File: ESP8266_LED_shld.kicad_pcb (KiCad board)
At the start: 2 copper layers, 59.1 x 52.7 mm, 29 parts, among them J1 Pwr_Dat_Out, J2 CONN_02X08, J3 CONN_DIN, J4 BARREL_JACK, J5 USB-MICROB, J6 CONN_01X06, M1 LOGIC_LEVEL_CONVERTER, T1 Test_Point_2Pads, U1 ESP-07v2, U2 AMS1117

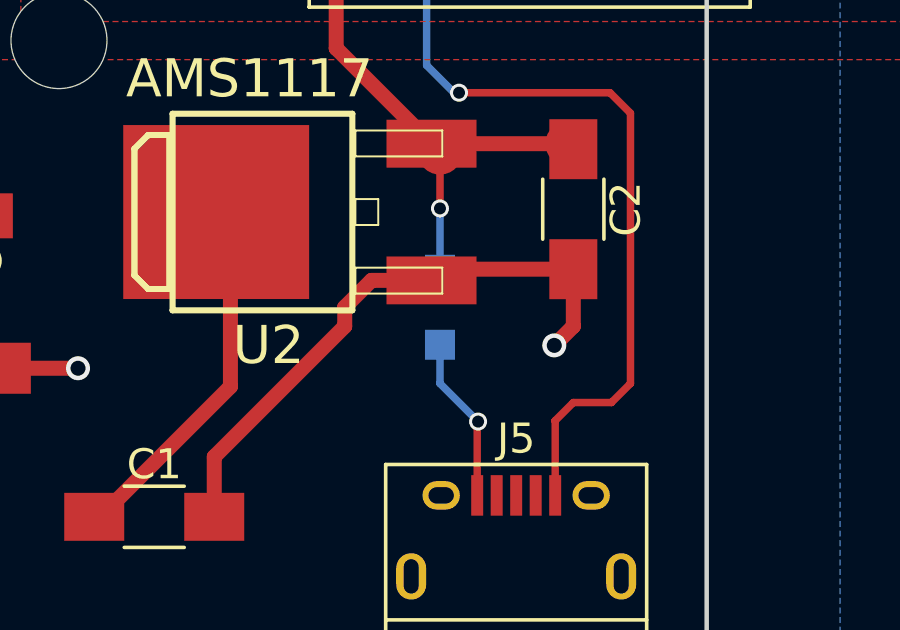
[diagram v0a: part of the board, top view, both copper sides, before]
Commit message: updated PCB design
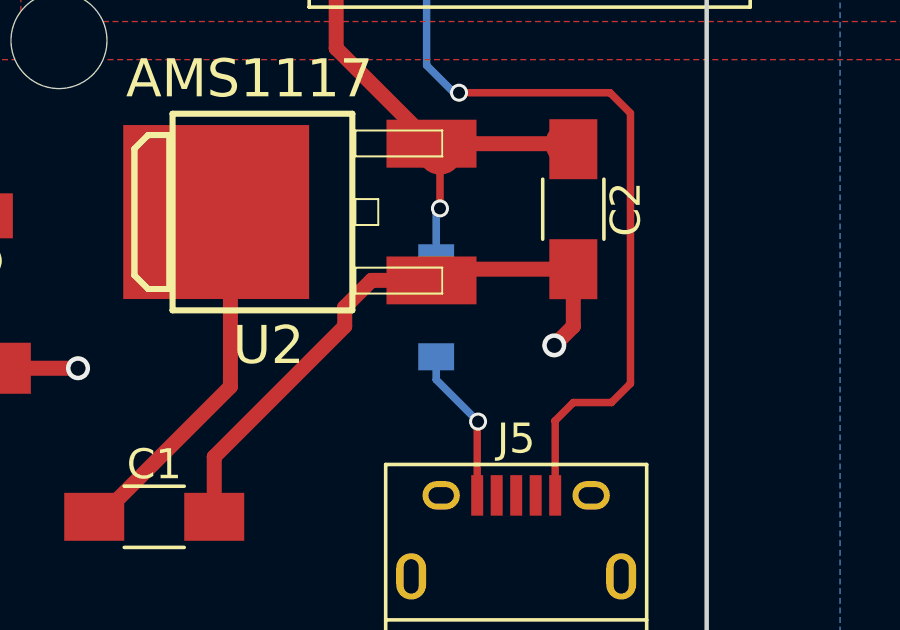
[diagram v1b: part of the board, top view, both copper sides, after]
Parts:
- D2: footprint Diodes_SMD:D_SOD-323_HandSoldering -> Diodes_SMD:D_SOD-123
- moved D2 0.13 mm to (208.8, 121.9)
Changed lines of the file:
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@@
     (thickness 1.6)
     (drawings 27)
-    (tracks 250)
+    (tracks 251)
     (zones 0)
     (modules 29)
@@
     )
   )
-  (module Diodes_SMD:D_SOD-323_HandSoldering (layer B.Cu)
-    (at 208.915 121.92 270)
-    (descr SOD-323)
-    (tags SOD-323)
-    (attr smd)
-    (fp_text reference D2 (at 0 1.85 270) (layer B.SilkS)
-      (effects (font (size 1 1) (thickness 0.15)) (justify mirror))
-    )
-    (fp_text value DIODE (at 0.1 -1.9 270) (layer B.Fab)
-      (effects (font (size 1 1) (thickness 0.15)) (justify mirror))
-    )
-    (fp_line (start -1.9 0.85) (end -1.9 -0.85) (layer B.SilkS) (width 0.12))
-    (fp_line (start 0.2 0) (end 0.45 0) (layer B.Fab) (width 0.1))
-    (fp_line (start 0.2 -0.35) (end -0.3 0) (layer B.Fab) (width 0.1))
-    (fp_line (start 0.2 0.35) (end 0.2 -0.35) (layer B.Fab) (width 0.1))
-    (fp_line (start -0.3 0) (end 0.2 0.35) (layer B.Fab) (width 0.1))
-    (fp_line (start -0.3 0) (end -0.5 0) (layer B.Fab) (width 0.1))
-    (fp_line (start -0.3 0.35) (end -0.3 -0.35) (layer B.Fab) (width 0.1))
-    (fp_line (start -0.9 -0.7) (end -0.9 0.7) (layer B.Fab) (width 0.1))
-    (fp_line (start 0.9 -0.7) (end -0.9 -0.7) (layer B.Fab) (width 0.1))
-    (fp_line (start 0.9 0.7) (end 0.9 -0.7) (layer B.Fab) (width 0.1))
-    (fp_line (start -0.9 0.7) (end 0.9 0.7) (layer B.Fab) (width 0.1))
-    (fp_line (start -2 0.95) (end 2 0.95) (layer B.CrtYd) (width 0.05))
-    (fp_line (start 2 0.95) (end 2 -0.95) (layer B.CrtYd) (width 0.05))
-    (fp_line (start -2 -0.95) (end 2 -0.95) (layer B.CrtYd) (width 0.05))
-    (fp_line (start -2 0.95) (end -2 -0.95) (layer B.CrtYd) (width 0.05))
-    (fp_line (start -1.9 -0.85) (end 1.25 -0.85) (layer B.SilkS) (width 0.12))
-    (fp_line (start -1.9 0.85) (end 1.25 0.85) (layer B.SilkS) (width 0.12))
-    (pad 1 smd rect (at -1.25 0 270) (size 1 1) (layers B.Cu B.Paste B.Mask)
-      (net 1 Vin))
-    (pad 2 smd rect (at 1.25 0 270) (size 1 1) (layers B.Cu B.Paste B.Mask)
-      (net 30 "Net-(D2-Pad2)"))
-    (model Diodes_SMD.3dshapes/D_SOD-323.wrl
-      (at (xyz 0 0 0))
-      (scale (xyz 1 1 1))
-      (rotate (xyz 0 0 180))
-    )
-  )
   (module Capacitors_SMD:CP_Elec_8x10 (layer F.Cu)
     (at 196.85 104.14 180)
@@
     )
   )
+  (module Diodes_SMD:D_SOD-123 (layer B.Cu)
+    (at 208.788 121.92 270)
+    (descr SOD-123)
+    (tags SOD-123)
+    (attr smd)
+    (fp_text reference D2 (at 0 2 270) (layer B.SilkS)
+      (effects (font (size 1 1) (thickness 0.15)) (justify mirror))
+    )
+    (fp_text value DIODE (at 0 -2.1 270) (layer B.Fab)
+      (effects (font (size 1 1) (thickness 0.15)) (justify mirror))
+    )
+    (fp_line (start -2.25 1) (end -2.25 -1) (layer B.SilkS) (width 0.12))
+    (fp_line (start 0.25 0) (end 0.75 0) (layer B.Fab) (width 0.1))
+    (fp_line (start 0.25 -0.4) (end -0.35 0) (layer B.Fab) (width 0.1))
+    (fp_line (start 0.25 0.4) (end 0.25 -0.4) (layer B.Fab) (width 0.1))
+    (fp_line (start -0.35 0) (end 0.25 0.4) (layer B.Fab) (width 0.1))
+    (fp_line (start -0.35 0) (end -0.35 -0.55) (layer B.Fab) (width 0.1))
+    (fp_line (start -0.35 0) (end -0.35 0.55) (layer B.Fab) (width 0.1))
+    (fp_line (start -0.75 0) (end -0.35 0) (layer B.Fab) (width 0.1))
+    (fp_line (start -1.4 -0.9) (end -1.4 0.9) (layer B.Fab) (width 0.1))
+    (fp_line (start 1.4 -0.9) (end -1.4 -0.9) (layer B.Fab) (width 0.1))
+    (fp_line (start 1.4 0.9) (end 1.4 -0.9) (layer B.Fab) (width 0.1))
+    (fp_line (start -1.4 0.9) (end 1.4 0.9) (layer B.Fab) (width 0.1))
+    (fp_line (start -2.35 1.15) (end 2.35 1.15) (layer B.CrtYd) (width 0.05))
+    (fp_line (start 2.35 1.15) (end 2.35 -1.15) (layer B.CrtYd) (width 0.05))
+    (fp_line (start 2.35 -1.15) (end -2.35 -1.15) (layer B.CrtYd) (width 0.05))
+    (fp_line (start -2.35 1.15) (end -2.35 -1.15) (layer B.CrtYd) (width 0.05))
+    (fp_line (start -2.25 -1) (end 1.65 -1) (layer B.SilkS) (width 0.12))
+    (fp_line (start -2.25 1) (end 1.65 1) (layer B.SilkS) (width 0.12))
+    (pad 1 smd rect (at -1.65 0 270) (size 0.9 1.2) (layers B.Cu B.Paste B.Mask)
+      (net 1 Vin))
+    (pad 2 smd rect (at 1.65 0 270) (size 0.9 1.2) (layers B.Cu B.Paste B.Mask)
+      (net 30 "Net-(D2-Pad2)"))
+    (model ${KISYS3DMOD}/Diodes_SMD.3dshapes/D_SOD-123.wrl
+      (at (xyz 0 0 0))
+      (scale (xyz 1 1 1))
+      (rotate (xyz 0 0 0))
+    )
+  )
   (gr_text "EN\n\n\n\nDIS" (at 163.322 124.46) (layer F.SilkS)
     (effects (font (size 0.76 0.6) (thickness 0.125)) (justify left))
@@
   (gr_line (start 217.805 133.35) (end 165.1 133.35) (layer Edge.Cuts) (width 0.15))
   (gr_line (start 217.805 86.995) (end 217.805 133.35) (layer Edge.Cuts) (width 0.15))
+  (segment (start 208.788 120.27) (end 208.788 118.751548) (width 0.25) (layer B.Cu) (net 1))
+  (via (at 208.915 118.624548) (size 0.6) (drill 0.4) (layers F.Cu B.Cu) (net 1))
   (segment (start 208.915 118.624548) (end 208.915 116.74856) (width 0.25) (layer F.Cu) (net 1))
-  (via (at 208.915 118.624548) (size 0.6) (drill 0.4) (layers F.Cu B.Cu) (net 1))
-  (segment (start 208.915 120.67) (end 208.915 118.624548) (width 0.25) (layer B.Cu) (net 1))
+  (segment (start 208.788 118.751548) (end 208.915 118.624548) (width 0.25) (layer B.Cu) (net 1))
   (segment (start 208.915 116.74856) (end 208.63306 116.46662) (width 1.5) (layer F.Cu) (net 1))
   (segment (start 208.63306 116.46662) (end 213.17662 116.46662) (width 0.5) (layer F.Cu) (net 1))
@@
   (segment (start 190.628 118.872) (end 190.628 123.602) (width 0.25) (layer F.Cu) (net 29))
   (segment (start 190.628 123.602) (end 190.278 123.952) (width 0.25) (layer F.Cu) (net 29))
+  (segment (start 208.788 123.57) (end 208.788 124.333) (width 0.25) (layer B.Cu) (net 30))
+  (segment (start 208.788 124.333) (end 210.185 125.73) (width 0.25) (layer B.Cu) (net 30))
   (segment (start 210.155 128.19) (end 210.155 125.76) (width 0.25) (layer F.Cu) (net 30))
   (segment (start 210.155 125.76) (end 210.185 125.73) (width 0.25) (layer F.Cu) (net 30))
-  (segment (start 210.185 125.73) (end 208.915 124.46) (width 0.25) (layer B.Cu) (net 30))
   (via (at 210.185 125.73) (size 0.6) (drill 0.4) (layers F.Cu B.Cu) (net 30))
   (segment (start 210.15706 125.75794) (end 210.185 125.73) (width 0.25) (layer F.Cu) (net 30))
-  (segment (start 208.915 124.46) (end 208.915 123.17) (width 0.25) (layer B.Cu) (net 30))
   (segment (start 202.735 85.852) (end 204.724 85.852) (width 0.25) (layer B.Cu) (net 33))
   (segment (start 200.025 97.155) (end 198.647219 95.777219) (width 0.25) (layer B.Cu) (net 33))
